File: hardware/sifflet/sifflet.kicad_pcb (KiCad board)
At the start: 2 copper layers, 0 parts

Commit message: PCB mechanical validation
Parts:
- added BT1: Battery, Battery:BatteryHolder_Keystone_3008_1x2450, B.Cu at (151.5, 120.5)
- added G***: LOGO, 0_stimulu-common:sinestimulus_logo, F.Cu at (151.5, 126.5)
- added J1: CX70M-24P1, 0_stimulu-common:USB-C_Female_CX70M-24P1, F.Cu at (178.0, 111.5)
- added REF**: POT_ALPS_RK08H1120_RK08H1220_B2B_short, 0_stimulu-common:POT_ALPS_RK08H1120_RK08H1220_B2B_short, F.Cu at (151.5, 144.5)
- added REF**: POT_ALPS_RK08H1120_RK08H1220_B2B_short, 0_stimulu-common:POT_ALPS_RK08H1120_RK08H1220_B2B_short, F.Cu at (122.9, 128.0)
- added REF**: HOPERF_RFM9XW_SMD, RF_Module:HOPERF_RFM9XW_SMD, F.Cu at (152.2, 111.5)
- added REF**: order_number, 0_stimulu-common:order_number, F.Cu at (151.5, 111.5)
- added REF**: POT_ALPS_RK08H1120_RK08H1220_B2B, 0_stimulu-common:POT_ALPS_RK08H1120_RK08H1220_B2B, F.Cu at (122.3, 111.5)
- added REF**: POT_ALPS_RK08H1120_RK08H1220_B2B, 0_stimulu-common:POT_ALPS_RK08H1120_RK08H1220_B2B, F.Cu at (136.9, 136.8)
- added REF**: POT_ALPS_RK08H1120_RK08H1220_B2B, 0_stimulu-common:POT_ALPS_RK08H1120_RK08H1220_B2B, F.Cu at (166.1, 136.8)
- added REF**: SW_SPST_B3U-3000P-B, Button_Switch_SMD:SW_SPST_B3U-3000P-B, F.Cu at (136.4, 85.5)
- added REF**: MountingHole_2.2mm_M2_Pad, MountingHole:MountingHole_2.2mm_M2_Pad, F.Cu at (122.1, 99.9)
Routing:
- added copper zone on B.Cu, net Net-(J1-PadSH)
- added copper zone on F.Cu, net Net-(J1-PadSH)
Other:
- board outline added: 64.5 x 72.1 mm
- board text added: "190509 REV 1"
- board text added: "SIFFLET mechanical validation"

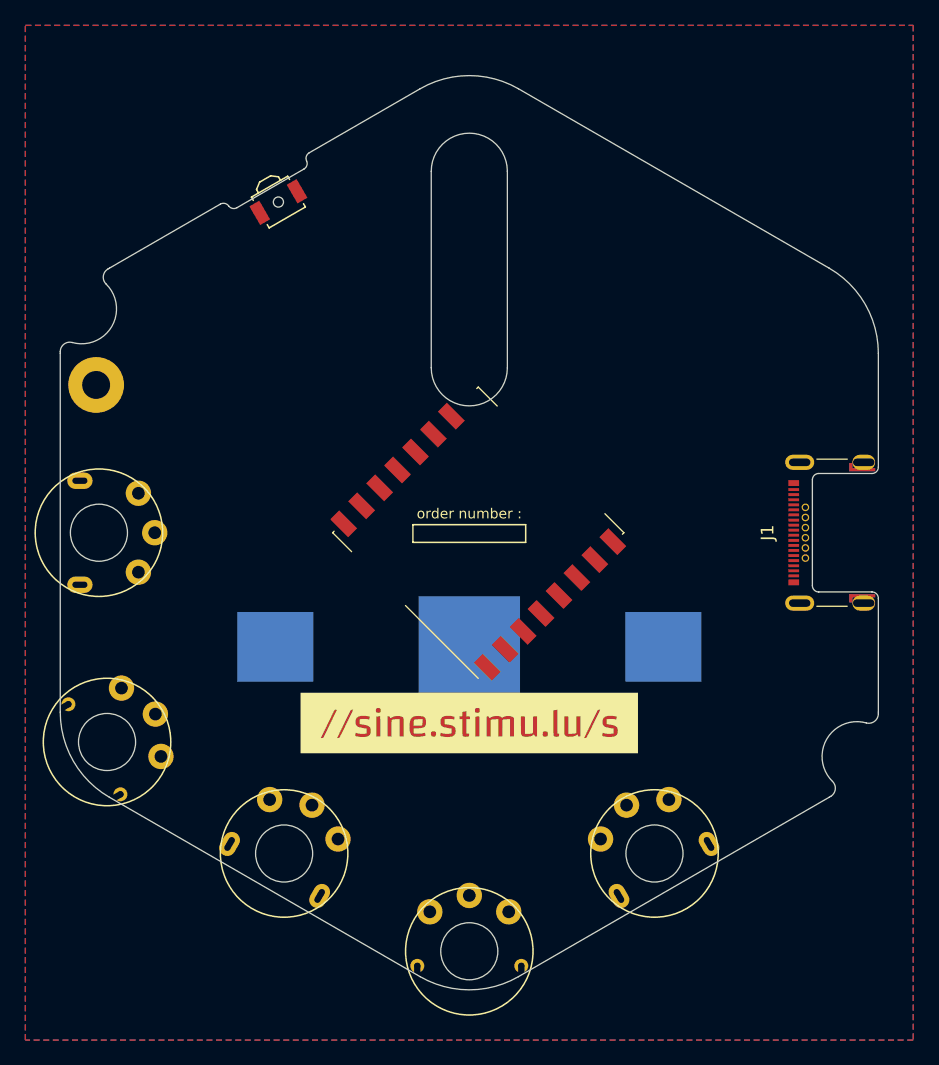
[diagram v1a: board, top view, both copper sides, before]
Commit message: CHanges for july 2019
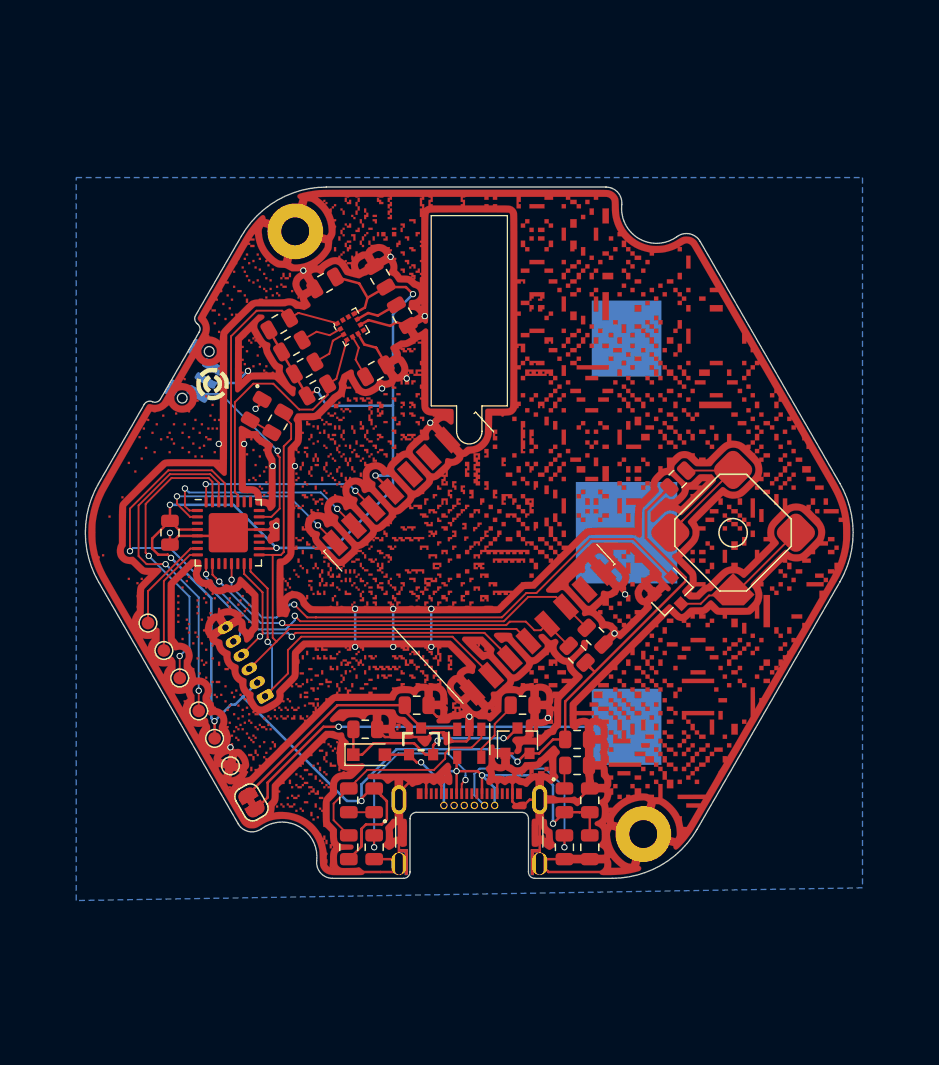
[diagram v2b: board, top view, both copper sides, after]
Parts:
- removed the G*** at (151.5, 126.5)
- removed the REF** at (151.5, 144.5)
- removed the REF** at (122.9, 128.0)
- removed the REF** at (152.2, 111.5)
- removed the REF** at (151.5, 111.5)
- removed the REF** at (122.3, 111.5)
- removed the REF** at (136.9, 136.8)
- removed the REF** at (166.1, 136.8)
- removed the REF** at (136.4, 85.5)
- removed the REF** at (122.1, 99.9)
- added BZ1: Buzzer, 0_stimulu-common:KSSG74B16_BUZZER, F.Cu at (172.3, 111.5)
- added C1: 0.1µF, Capacitor_SMD:C_0805_2012Metric, F.Cu at (127.9, 111.5)
- added C2: 0.1µF, Capacitor_SMD:C_0805_2012Metric, F.Cu at (144.1, 98.8)
- added C3: 0.1µf, Capacitor_SMD:C_0805_2012Metric, F.Cu at (144.5, 91.4)
- added C4: 0.1µF, Capacitor_SMD:C_0805_2012Metric, F.Cu at (146.2, 94.4)
- added C5: 10µF, Capacitor_SMD:C_0805_2012Metric, F.Cu at (140.1, 91.8)
- added C6: 4.7µF, Capacitor_SMD:C_0805_2012Metric, F.Cu at (161.0, 132.6)
- added C7: 4.7µF, Capacitor_SMD:C_0805_2012Metric, F.Cu at (147.3, 125.1)
- added C8: 4.7µF, Capacitor_SMD:C_0805_2012Metric, F.Cu at (143.3, 127.0)
- added C9: 1µF, Capacitor_SMD:C_0805_2012Metric, F.Cu at (160.0, 127.8)
- added D1: ON, 0_stimulu-common:LED_0805_2012Metric, F.Cu at (159.0, 132.6)
- added D2: LED_CTRL, 0_stimulu-common:LED_0805_2012Metric, F.Cu at (134.7, 101.8)
- added D3: CHARGING, 0_stimulu-common:LED_0805_2012Metric, F.Cu at (144.0, 132.6)
- added D4: BAT60JFILM, Diode_SMD:D_SOD-323_HandSoldering, F.Cu at (143.6, 129.0)
- added G***: LOGO, 0_stimulu-common:SYMBOL_SIFFLET, F.Cu at (131.4, 99.7)
- added G***: LOGO, 0_stimulu-common:MOTIF_SIFFLET, F.Cu at (151.5, 111.5)
- added G***: LOGO, 0_stimulu-common:MASK_SIFFLET, F.Cu at (153.9, 113.3)
- added H1: MountingHole_Pad, MountingHole:MountingHole_2.2mm_M2_Pad, F.Cu at (137.8, 87.8)
- added H2: MountingHole_Pad, MountingHole:MountingHole_2.2mm_M2_Pad, F.Cu at (165.2, 135.3)
- added J2: ICSP header, Connector_Molex:Molex_PicoBlade_53048-0610_1x06_P1.25mm_Horizontal, B.Cu at (135.4, 124.4)
- added JP1: Current test point, Jumper:SolderJumper-2_P1.3mm_Bridged_RoundedPad1.0x1.5mm, F.Cu at (134.3, 132.8)
- added Q1: BSS138, Package_TO_SOT_SMD:SOT-23, F.Cu at (167.5, 116.4)
- added Q2: DMP1045U, procsynth:SOT23_FET, F.Cu at (147.7, 128.0)
- added R1: 5K1 PULLDOWN, Resistor_SMD:R_0805_2012Metric, F.Cu at (159.0, 136.3)
- added R10: 10K, Resistor_SMD:R_0805_2012Metric, F.Cu at (160.0, 121.1)
- added R11: 10K, Resistor_SMD:R_0805_2012Metric, F.Cu at (161.4, 119.7)
- added R12: R_Small, Resistor_SMD:R_0805_2012Metric, F.Cu at (167.9, 107.3)
- added R13: 10K CALIB CHRG, Resistor_SMD:R_0805_2012Metric, F.Cu at (155.7, 125.1)
- added R14: 100K CHRG INIT LOAD, Resistor_SMD:R_0805_2012Metric, F.Cu at (161.0, 136.3)
- added R15: 47K PULLUP 3V, Resistor_SMD:R_0805_2012Metric, F.Cu at (142.0, 136.3)
- added R2: 5K1 PULLDOWN, Resistor_SMD:R_0805_2012Metric, F.Cu at (144.0, 136.3)
- added R3: 470, Resistor_SMD:R_0805_2012Metric, F.Cu at (160.0, 129.9)
- added R4: 1K I2C PULLUP, Resistor_SMD:R_0805_2012Metric, F.Cu at (139.5, 100.3)
- added R5: 10K CS_PULLUP, Resistor_SMD:R_0805_2012Metric, F.Cu at (137.5, 96.8)
- added R6: 10K CS_PULLUP, Resistor_SMD:R_0805_2012Metric, F.Cu at (138.5, 98.5)
- added R7: 1K, Resistor_SMD:R_0805_2012Metric, F.Cu at (136.4, 102.8)
- added R8: 1K1 I2C PULLUP, Resistor_SMD:R_0805_2012Metric, F.Cu at (136.5, 95.1)
- added R9: 470, Resistor_SMD:R_0805_2012Metric, F.Cu at (142.0, 132.6)
- added REF**: SIFFLET_OUTLINES, 0_stimulu-common:SIFFLET_OUTLINES, F.Cu at (151.5, 111.5)
- added SW1: SW_Push, 0_stimulu-common:TL3340_SWITCH_SMD, B.Cu at (129.9, 99.1)
- added TP1: GND, TestPoint:TestPoint_Pad_D1.0mm, F.Cu at (132.7, 129.9)
- added TP2: VCC, TestPoint:TestPoint_Pad_D1.0mm, F.Cu at (131.4, 127.7)
- added TP3: RX, TestPoint:TestPoint_Pad_D1.0mm, F.Cu at (130.2, 125.6)
- added TP4: XTAL1, TestPoint:TestPoint_Pad_D1.0mm, F.Cu at (126.2, 118.7)
- added TP5: TX, TestPoint:TestPoint_Pad_D1.0mm, F.Cu at (128.7, 123.0)
- added TP6: XTAL2, TestPoint:TestPoint_Pad_D1.0mm, F.Cu at (127.4, 120.8)
- added U1: ATmega328PB-MU, Package_DFN_QFN:QFN-32-1EP_5x5mm_P0.5mm_EP3.1x3.1mm, F.Cu at (132.5, 111.5)
- added U2: LSM303C, 0_stimulu-digikey:LGA-12_9x9mm_LSM303C, F.Cu at (142.1, 95.3)
- added U3: RFM95W-868S2, RF_Module:HOPERF_RFM9XW_SMD, F.Cu at (151.5, 113.5)
- added U4: MCP73831-2-OT, Package_TO_SOT_SMD:SOT-23-5, F.Cu at (151.5, 128.1)
- added U5: MCP1700-3302E_SOT23, Package_TO_SOT_SMD:SOT-23, F.Cu at (155.3, 127.9)
- BT1: value Battery -> Battery LIR2450
- moved J1 34.1 mm to (151.5, 133.0), turned to 0 degrees
- moved BT1 15.3 mm to (163.9, 111.5), turned to 270 degrees
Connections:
- BT1 pad 1: (no net) -> /V_LIPO
- BT1 pad 2: (no net) -> GND
- J1 pad A1: (no net) -> GND
- J1 pad A12: (no net) -> GND
- J1 pad A4: (no net) -> /V_USB
- J1 pad A5: (no net) -> Net-(J1-PadA5)
- J1 pad A9: (no net) -> /V_USB
- J1 pad B1: (no net) -> GND
- J1 pad B12: (no net) -> GND
- J1 pad B4: (no net) -> /V_USB
- J1 pad B5: (no net) -> Net-(J1-PadB5)
- J1 pad B9: (no net) -> /V_USB
- J1 pad SH: Net-(J1-PadSH) -> GND
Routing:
- net VCC: track 0.00 -> 166.3 mm, vias 0 -> 9
- net GND: track 0.00 -> 108.3 mm, vias 0 -> 25
- net /Digital_13: track 0.00 -> 44.9 mm
- net /Digital_9: track 0.00 -> 42.2 mm, vias 0 -> 2
- net /Digital_5: track 0.00 -> 35.4 mm, vias 0 -> 2
- net /Digital_12: track 0.00 -> 33.4 mm, vias 0 -> 1
- net /V_LIPO: track 0.00 -> 32.6 mm, vias 0 -> 1
- net /V_USB: track 0.00 -> 32.4 mm, vias 0 -> 4
- net /Digital_6: track 0.00 -> 31.9 mm, vias 0 -> 2
- net /Digital_11: track 0.00 -> 29.4 mm, vias 0 -> 2
- net /Digital_0: track 0.00 -> 28.2 mm, vias 0 -> 2
- net /RST: track 0.00 -> 27.1 mm, vias 0 -> 1
- net /Digital_1: track 0.00 -> 23.4 mm, vias 0 -> 2
- net /A5: track 0.00 -> 22.7 mm
- net /A4: track 0.00 -> 22.0 mm
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- added copper zone on B.Cu, net GND
- removed copper zone on B.Cu, net Net-(J1-PadSH)
- removed copper zone on F.Cu, net Net-(J1-PadSH)
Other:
- board size 64.5 x 72.1 mm -> 60.5 x 54.5 mm
- net class Default: clearance 0.1 -> 0.1525
- net class POWER: clearance 0.5 -> 0.1525; trace_width 0.5 -> 0.2
- rule trace_clearance: 0.1 -> 0.1525
- board text removed: "190509 REV 1"
- board text removed: "SIFFLET mechanical validation"
